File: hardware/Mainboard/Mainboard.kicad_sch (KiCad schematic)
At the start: 129 parts, among them CN1 NUCLE_F446RE_MORPHO_CN7, CN2 NUCLE_F446RE_MORPHO_CN10, J1 X_END, J10 Power, J12 Part_Cooling2, J13 Part_Cooling1, J2 Y_END, J27 Z_END, J28 X_MS2, J29 HE1_therm, J3 +12V, J30 Bed_therm, J31 Z1_MS2, J32 X_MS1, J33 Z1_MS1, J34 Z4_MS2, J35 Z4_MS1, J36 X_Motor, J37 Z1_Motor, J38 Y_MS2, J39 Z2_MS2, J40 Y_MS1, J41 Z2_MS1, J42 Z4_Motor, J43 Y_Motor, J44 Z2_Motor, J45 E_MS2, J46 Z3_MS2, J47 E_MS1, J48 Z3_MS1, J49 E_Motor, J50 Z3_Motor, J51 PWR_therm, J52 HE2_therm, J53 R_MS2, J54 R_MS1, J55 R_Motor, J6 Hotend1, J7 +24V, J8 Hotend2, J9 Bed, Q2 PSMN5R2-60YL, Q4 PSMN5R2-60YL, Q5 PSMN5R2-60YL, Q6 PSMN5R2-60YL, Q7 AO3400A, Q8 AO3400A, U1 MIC4426, U10 Z4, U11 Y, U12 Z2, U13 E, U14 Z3, U15 R, U2 MIC4426, U3 TPS54560BDDA, U4 MIC5219-3.3YM5, U8 X, U9 Z1

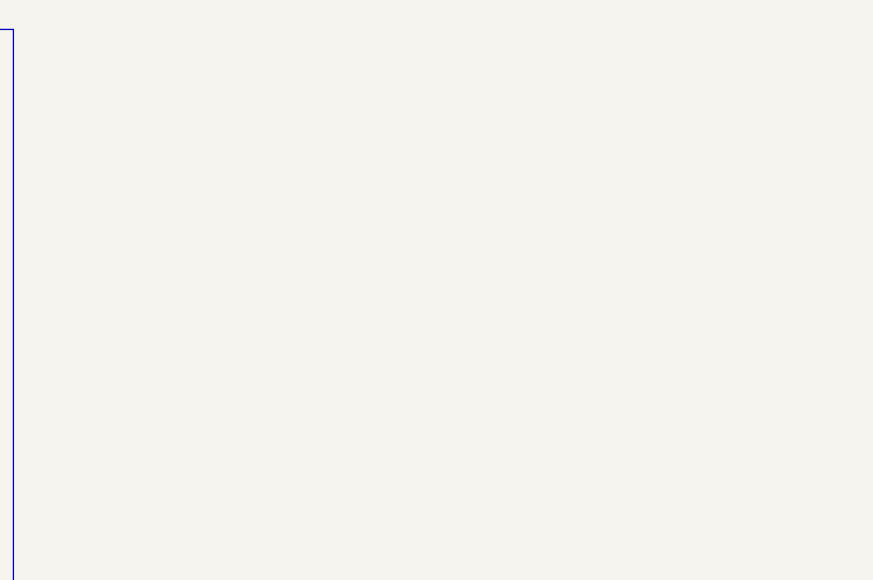
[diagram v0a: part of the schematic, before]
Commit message: mainboard v2
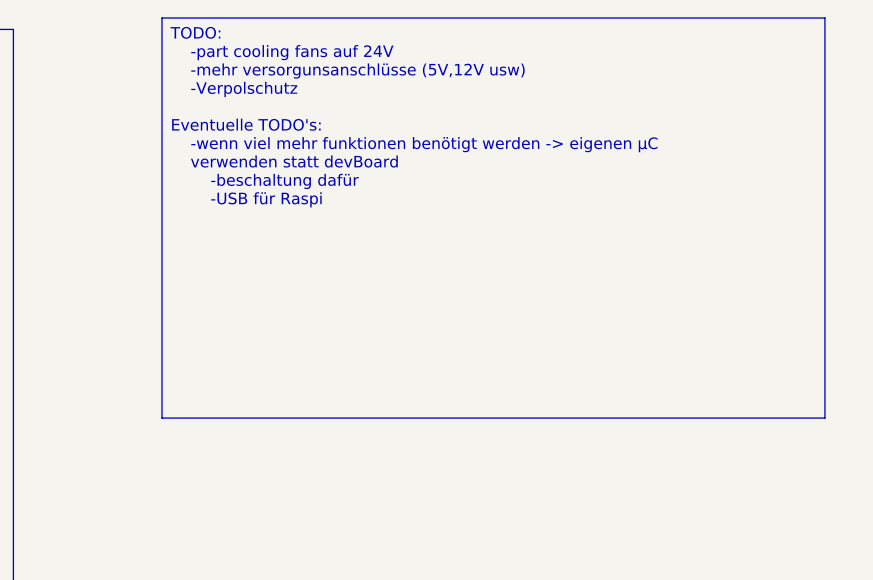
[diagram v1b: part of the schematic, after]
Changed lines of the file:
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@@
+		)
+	)
+	(text_box "TODO:\n	-part cooling fans auf 24V\n	-mehr versorgunsanschlüsse (5V,12V usw)\n	-Verpolschutz\n\nEventuelle TODO's:\n	-wenn viel mehr funktionen benötigt werden -> eigenen µC 	verwenden statt devBoard\n		-beschaltung dafür	\n		-USB für Raspi"
+		(exclude_from_sim no)
+		(at 422.91 12.7 0)
+		(size 73.66 44.45)
+		(margins 0.9525 0.9525 0.9525 0.9525)
+		(stroke
+			(width 0)
+			(type solid)
+		)
+		(fill
+			(type none)
+		)
+		(effects
+			(font
+				(size 1.27 1.27)
+			)
+			(justify left top)
 		)
 	)
